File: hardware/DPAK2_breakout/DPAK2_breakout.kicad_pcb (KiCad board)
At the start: 2 copper layers, 16.5 x 19.1 mm, 6 parts, among them P1 CONN_1, P2 CONN_2, P3 CONN_1, Q1 IRGS14C40L

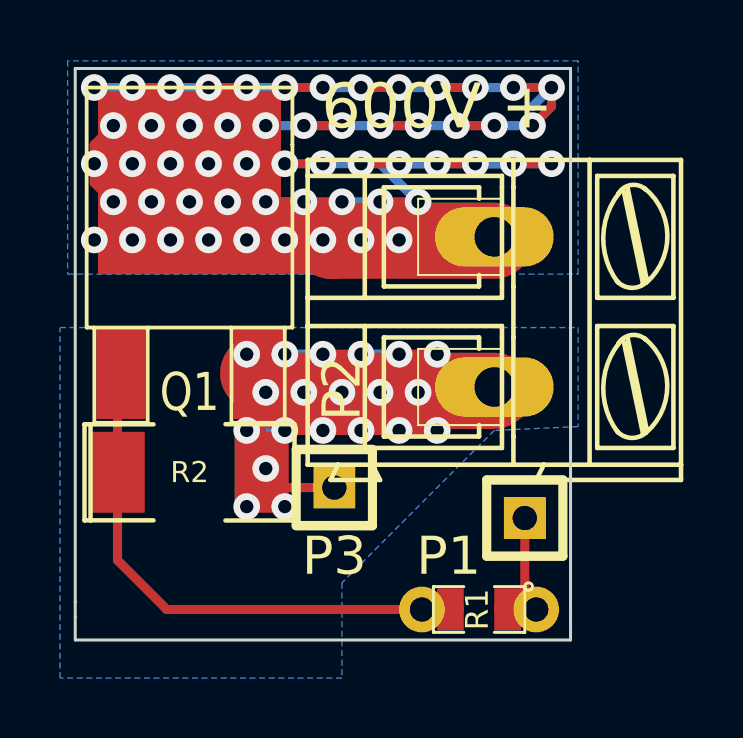
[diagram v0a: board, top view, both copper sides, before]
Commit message: update pcb files
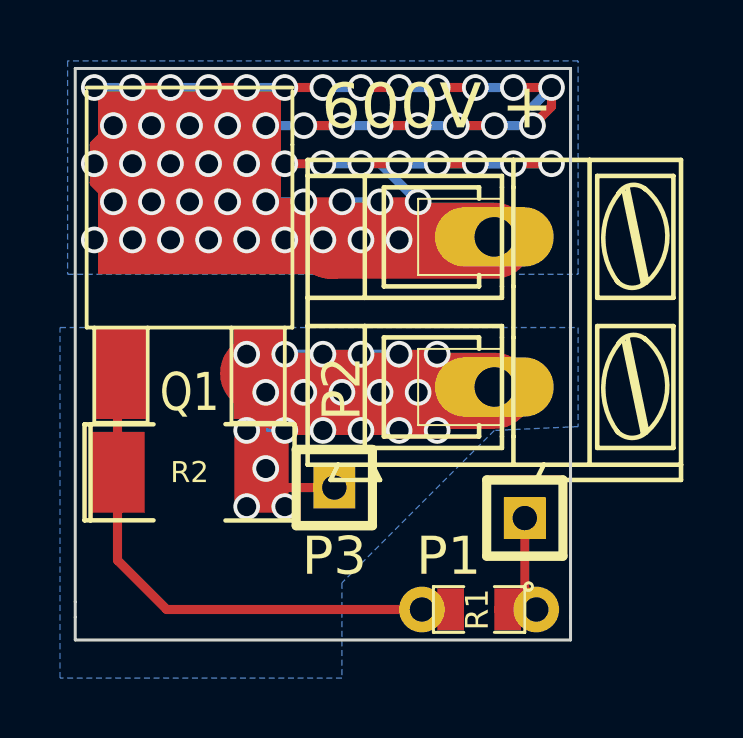
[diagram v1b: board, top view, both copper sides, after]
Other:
- net class Default removed
- net class FAT removed
- net class MIN removed
